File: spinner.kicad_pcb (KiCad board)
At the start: 2 copper layers, 147 x 147 mm, 114 parts, among them J1 Micro_SD_Card, SW1 SW_SPDT, U1 AP63205WU, U2 RS0102, U3 SFH617A-3X006, U4 SFH617A-3X006, U5 SFH617A-3X006, U6 ESP32-WROVER

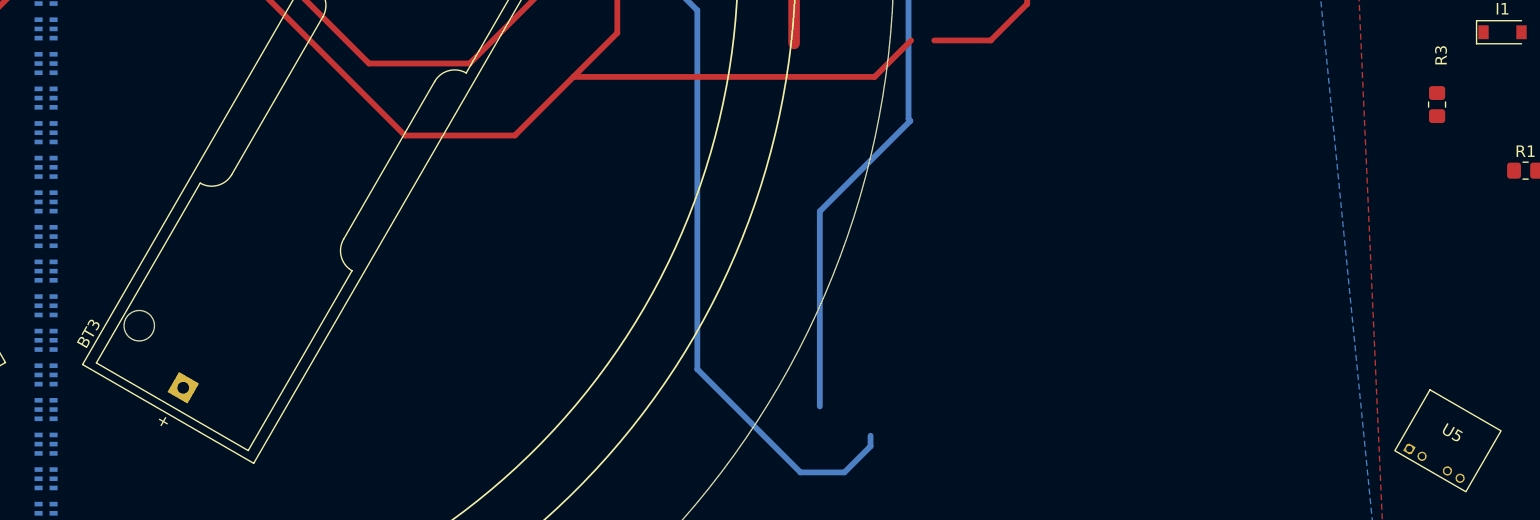
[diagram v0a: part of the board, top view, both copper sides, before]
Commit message: Moving all the version 9.0
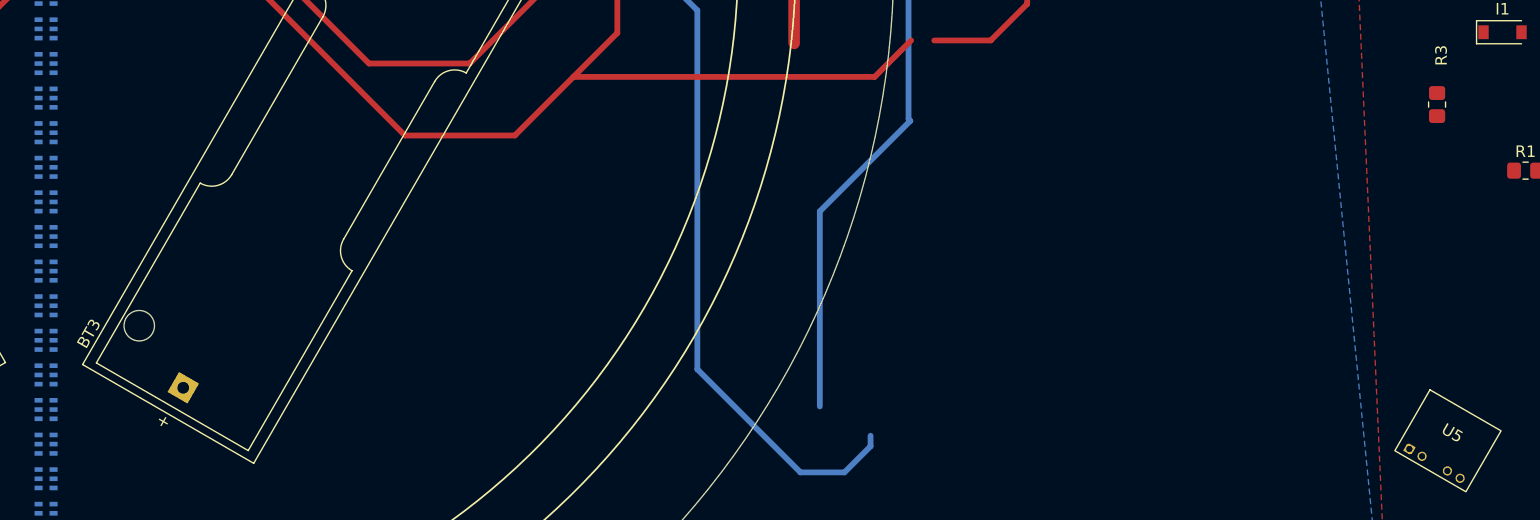
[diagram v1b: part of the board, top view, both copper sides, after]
